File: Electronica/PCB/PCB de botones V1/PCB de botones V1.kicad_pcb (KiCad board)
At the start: 2 copper layers, 80.3 x 28.4 mm, 14 parts, among them J2 Conn_02x05_Counter_Clockwise, SW2 SW_Push, SW4 SW_Push, SW9 SW_SPST

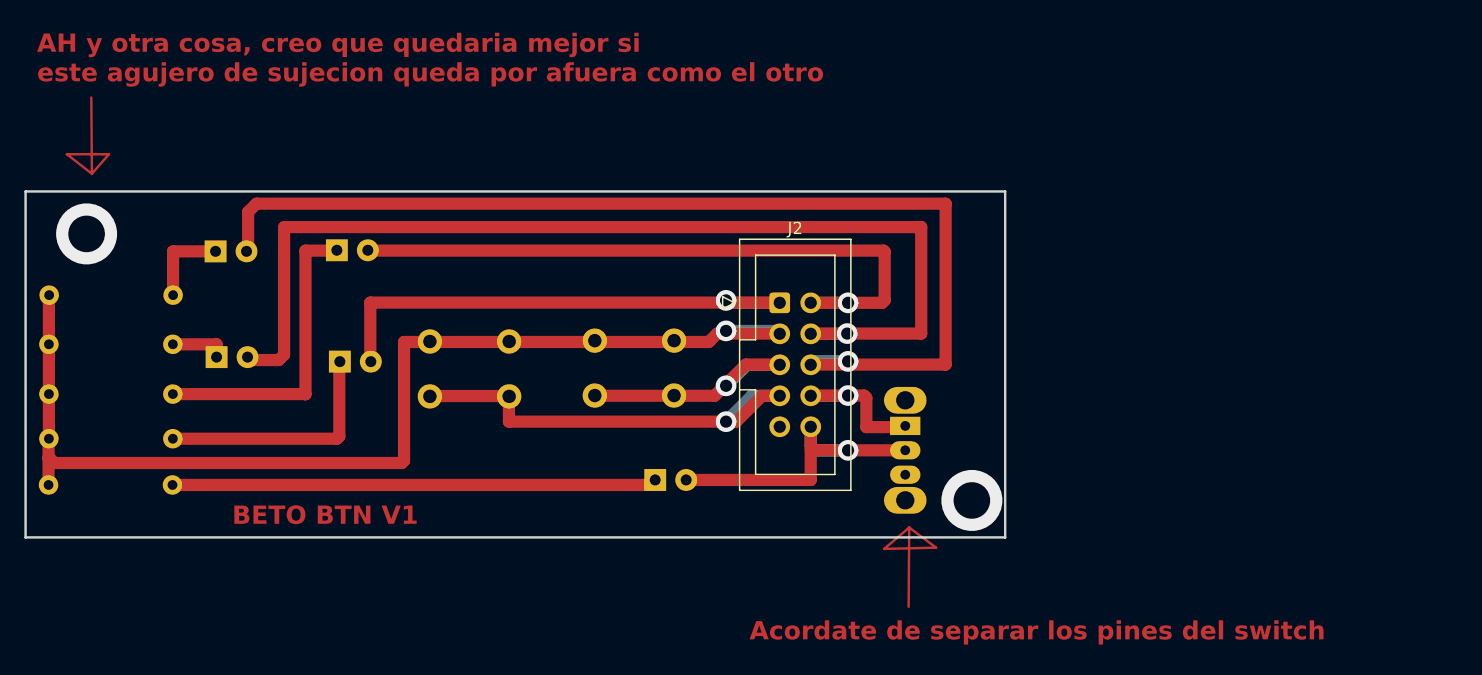
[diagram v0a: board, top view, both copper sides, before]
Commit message: pcb de leds
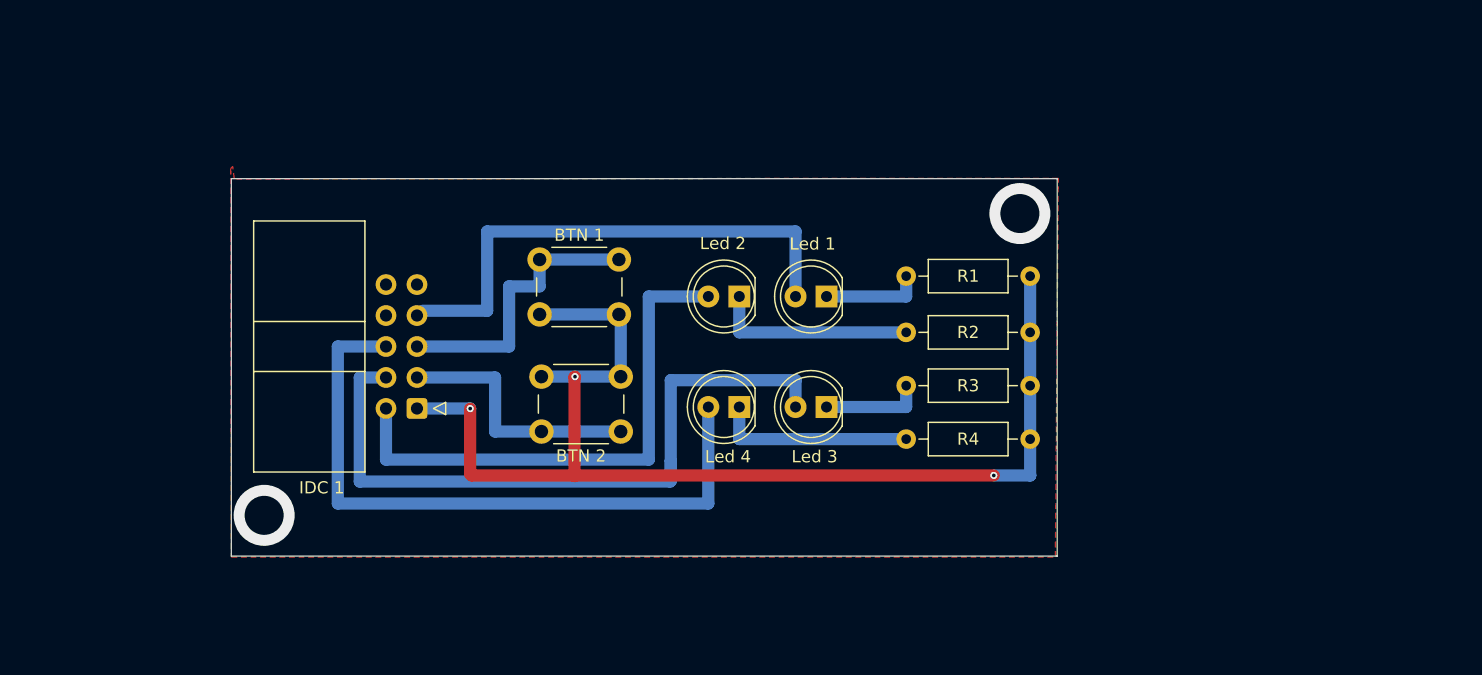
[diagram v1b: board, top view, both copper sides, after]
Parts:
- removed D10, D3, D7, D8, D9: LED, LED_THT:LED_D5.0mm
- removed J2: Conn_02x05_Counter_Clockwise, Connector_IDC:IDC-Header_2x05_P2.54mm_Vertical
- removed R10, R7, R8, R9: R_US, Resistor_THT:R_Axial_DIN0207_L6.3mm_D2.5mm_P10.16mm_Horizontal
- removed SW2, SW4: SW_Push, Button_Switch_THT:SW_PUSH_6mm
- removed SW9: SW_SPST, Button_Switch_THT:SW_Slide_SPDT_Straight_CK_OS102011MS2Q
- added BTN 1: SW_Push, Button_Switch_THT:SW_PUSH_6mm, F.Cu at (191.4, 80.1)
- added BTN 2: SW_Push, Button_Switch_THT:SW_PUSH_6mm, F.Cu at (198.1, 94.2)
- added IDC 1: IDC Placa Botones, Connector_IDC:IDC-Header_2x05_P2.54mm_Horizontal, F.Cu at (181.4, 92.3)
- added Led 1: LED, LED_THT:LED_D5.0mm, F.Cu at (215.0, 83.2)
- added Led 2: LED, LED_THT:LED_D5.0mm, F.Cu at (207.8, 83.2)
- added Led 3: LED, LED_THT:LED_D5.0mm, F.Cu at (215.0, 92.2)
- added Led 4: LED, LED_THT:LED_D5.0mm, F.Cu at (207.8, 92.2)
- added R1: R_US, Resistor_THT:R_Axial_DIN0207_L6.3mm_D2.5mm_P10.16mm_Horizontal, F.Cu at (231.7, 81.5)
- added R2: R_US, Resistor_THT:R_Axial_DIN0207_L6.3mm_D2.5mm_P10.16mm_Horizontal, F.Cu at (231.7, 86.1)
- added R4: R_US, Resistor_THT:R_Axial_DIN0207_L6.3mm_D2.5mm_P10.16mm_Horizontal, F.Cu at (231.7, 94.8)
- R3: moved to F.Cu
- moved R3 80.9 mm to (231.7, 90.5), turned to 180 degrees
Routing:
- net Net-(D7-A): track 88.2 -> 0.00 mm, vias 1 -> 0
- net Net-(D10-A): track 86.7 -> 0.00 mm, vias 1 -> 0
- net LED3: track 0.00 -> 58.0 mm
- net Net-(D9-A): track 55.5 -> 0.00 mm, vias 1 -> 0
- net LED4: track 0.00 -> 55.1 mm
- net LED2: track 0.00 -> 44.0 mm
- net Net-(D8-A): track 42.8 -> 0.00 mm, vias 1 -> 0
- net LED1: track 0.00 -> 42.4 mm
- net Net-(J2-Pin_7): track 37.0 -> 0.00 mm, vias 1 -> 0
- net Net-(D3-K): track 39.7 -> 8.28 mm
- net Net-(D3-A): track 27.1 -> 0.00 mm, vias 1 -> 0
- net Net-(D9-K): track 25.4 -> 0.00 mm
- net BTN1: track 0.00 -> 23.7 mm
- net BTN2: track 0.00 -> 21.1 mm
- net Net-(J2-Pin_5): track 21.1 -> 0.00 mm, vias 1 -> 0
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- added copper zone on F.Cu, net GND
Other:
- board size 80.3 x 28.4 mm -> 67.7 x 30.9 mm
- board text removed: "AH y otra cosa, creo que quedaria mejor si este agujero de sujecion queda por afuera como el otro"
- board text removed: "Acordate de separar los pines del switch"
- board text removed: "BETO BTN V1"
